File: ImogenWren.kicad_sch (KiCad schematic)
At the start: 16 parts, among them J1 WS2821_LED_OUT, SW1 Power, U1 MCP73831-2-OT

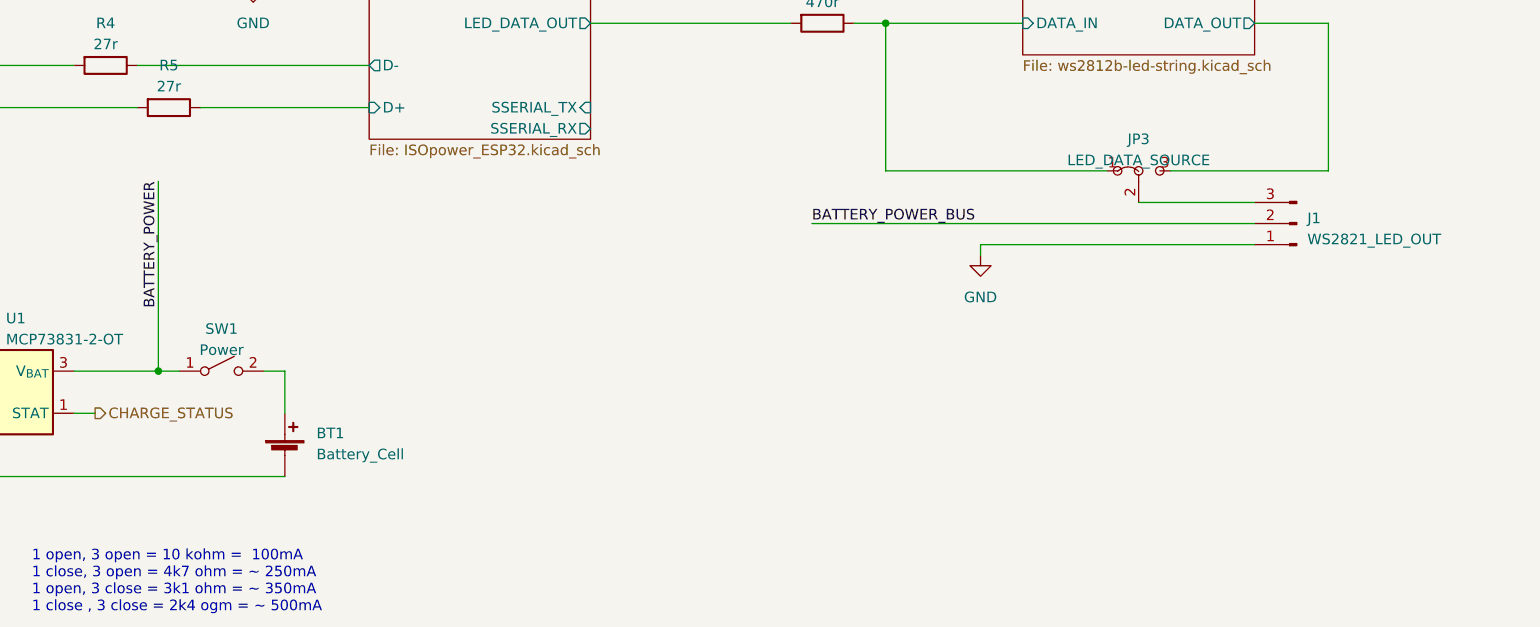
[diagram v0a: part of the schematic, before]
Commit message: xcfgdfgd
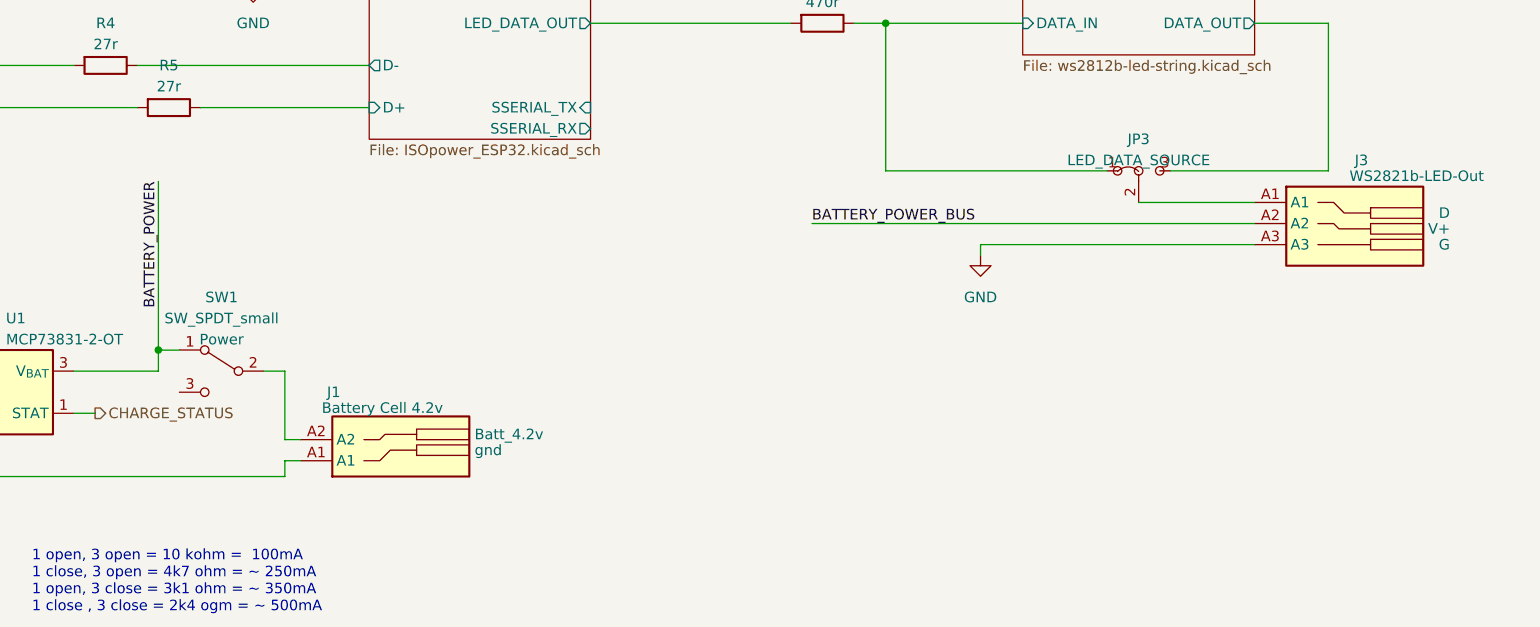
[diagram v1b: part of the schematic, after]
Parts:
- removed BT1: Battery_Cell, Battery:BatteryHolder_Keystone_1060_1x2032, symbol Device:Battery_Cell
- removed J1: WS2821_LED_OUT, Connector_PCBEdge:BUS_PCIexpress_x1, symbol 000_Connectors_Immo:3pin_molex_2.54mm_male
- removed SW1: Power, Button_Switch_SMD:SW_SPDT_PCM12, symbol Switch:SW_SPST
- added J1: Battery Cell 4.2v, 000-edge-connectors-immo:2-pin-edge, symbol 000-lost-edge-connectors:2-pin-edge-touch
- added J3: WS2821b-LED-Out, 000-edge-connectors-immo:3-pin-edge, symbol 000-lost-edge-connectors:3-pin-edge-touch
- added SW1: SW_SPDT_small, 000_Switches_Immo:SW_SPDT_PCM12, symbol 000_Switches_Immo:SW_SPDT_small
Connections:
- net BATTERY_POWER: now also SW1.1 (A)
- net BATTERY_POWER_BUS: now also J3.A2
- net GND: now also J3.A3
- net GNDPWR: now also J1.A1
- net at JP3.2 (C): now also J3.A1
- new net: J1.A2, SW1.2 (B)
